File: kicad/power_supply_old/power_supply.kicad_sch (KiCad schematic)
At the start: 0 parts

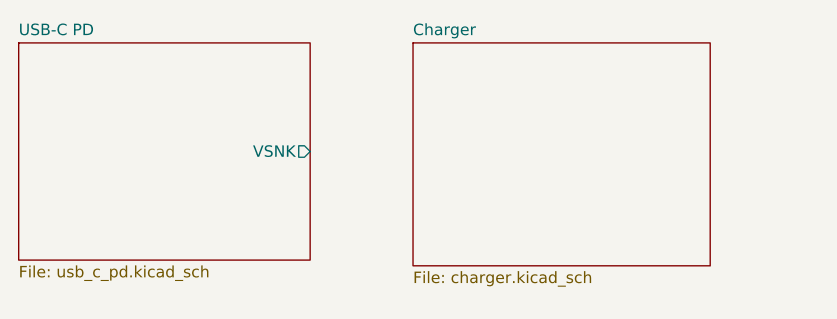
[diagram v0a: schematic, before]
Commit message: working on psu schematic capture
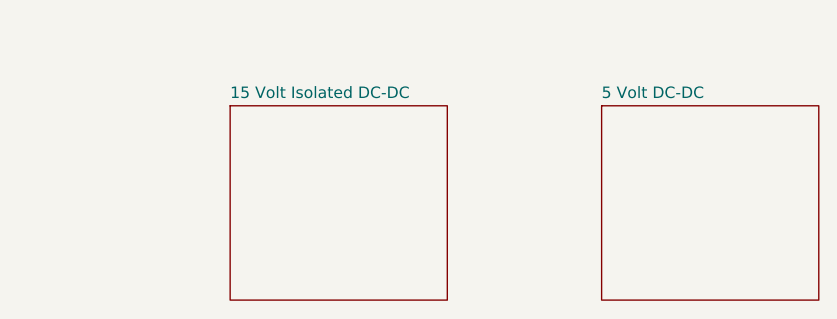
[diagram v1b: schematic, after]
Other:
- removed sheet Charger
- removed sheet USB-C PD
- added sheet 15 Volt Isolated DC-DC (isolated_dc_to_dc.kicad_sch)
- added sheet 5 Volt DC-DC (5_volt_dc_to_dc.kicad_sch)
- title: Power Supply -> Bidirectional Load Switch
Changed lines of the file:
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@@
 	(paper "A4")
 	(title_block
-		(title "Power Supply")
-		(date "2024-10-27")
-		(rev "0.1.0")
+		(title "Bidirectional Load Switch")
+		(date "2024-09-17")
+		(rev "0")
 		(company "University of Wisconsin-Platteville")
-		(comment 1 "Nicholas Loehrke")
 	)
 	(sheet
-		(at 88.265 41.275)
-		(size 33.02 24.765)
+		(at 67.945 48.26)
+		(size 24.13 21.59)
 		(fields_autoplaced yes)
 		(stroke
@@
 			(color 0 0 0 0.0000)
 		)
-		(property "Sheetname" "Charger"
-			(at 88.265 40.5634 0)
+		(property "Sheetname" "15 Volt Isolated DC-DC"
+			(at 67.945 47.5484 0)
 			(effects
 				(font
@@
 			)
 		)
-		(property "Sheetfile" "charger.kicad_sch"
-			(at 88.265 66.6246 0)
+		(property "Sheetfile" "isolated_dc_to_dc.kicad_sch"
+			(at 67.945 70.4346 0)
 			(effects
 				(font
@@
 				)
 				(justify left top)
+				(hide yes)
 			)
 		)
 		(instances
 			(project "power_supply"
-				(path "/6a7d9dc9-f78f-470f-911b-b95256023173"
-					(page "3")
+				(path "/a4768a02-c961-4971-939f-bbf2bfa51fa3"
+					(page "2")
 				)
 			)
@@
 	)
 	(sheet
-		(at 44.45 41.275)
-		(size 32.385 24.13)
+		(at 109.22 48.26)
+		(size 24.13 21.59)
 		(fields_autoplaced yes)
 		(stroke
@@
 			(color 0 0 0 0.0000)
 		)
-		(property "Sheetname" "USB-C PD"
-			(at 44.45 40.5634 0)
+		(property "Sheetname" "5 Volt DC-DC"
+			(at 109.22 47.5484 0)
 			(effects
 				(font
@@
 			)
 		)
-		(property "Sheetfile" "usb_c_pd.kicad_sch"
-			(at 44.45 65.9896 0)
+		(property "Sheetfile" "5_volt_dc_to_dc.kicad_sch"
+			(at 109.22 70.4346 0)
 			(effects
 				(font
@@
 				)
 				(justify left top)
-			)
-		)
-		(pin "VSNK" output
-			(at 76.835 53.34 0)
-			(effects
-				(font
-					(size 1.27 1.27)
-				)
-				(justify right)
+				(hide yes)
 			)
 		)
 		(instances
 			(project "power_supply"
-				(path "/6a7d9dc9-f78f-470f-911b-b95256023173"
-					(page "2")
+				(path "/a4768a02-c961-4971-939f-bbf2bfa51fa3"
+					(page "3")
 				)
 			)
